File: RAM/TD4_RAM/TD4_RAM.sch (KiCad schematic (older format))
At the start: 1 part, among them U1 74AHC1G32

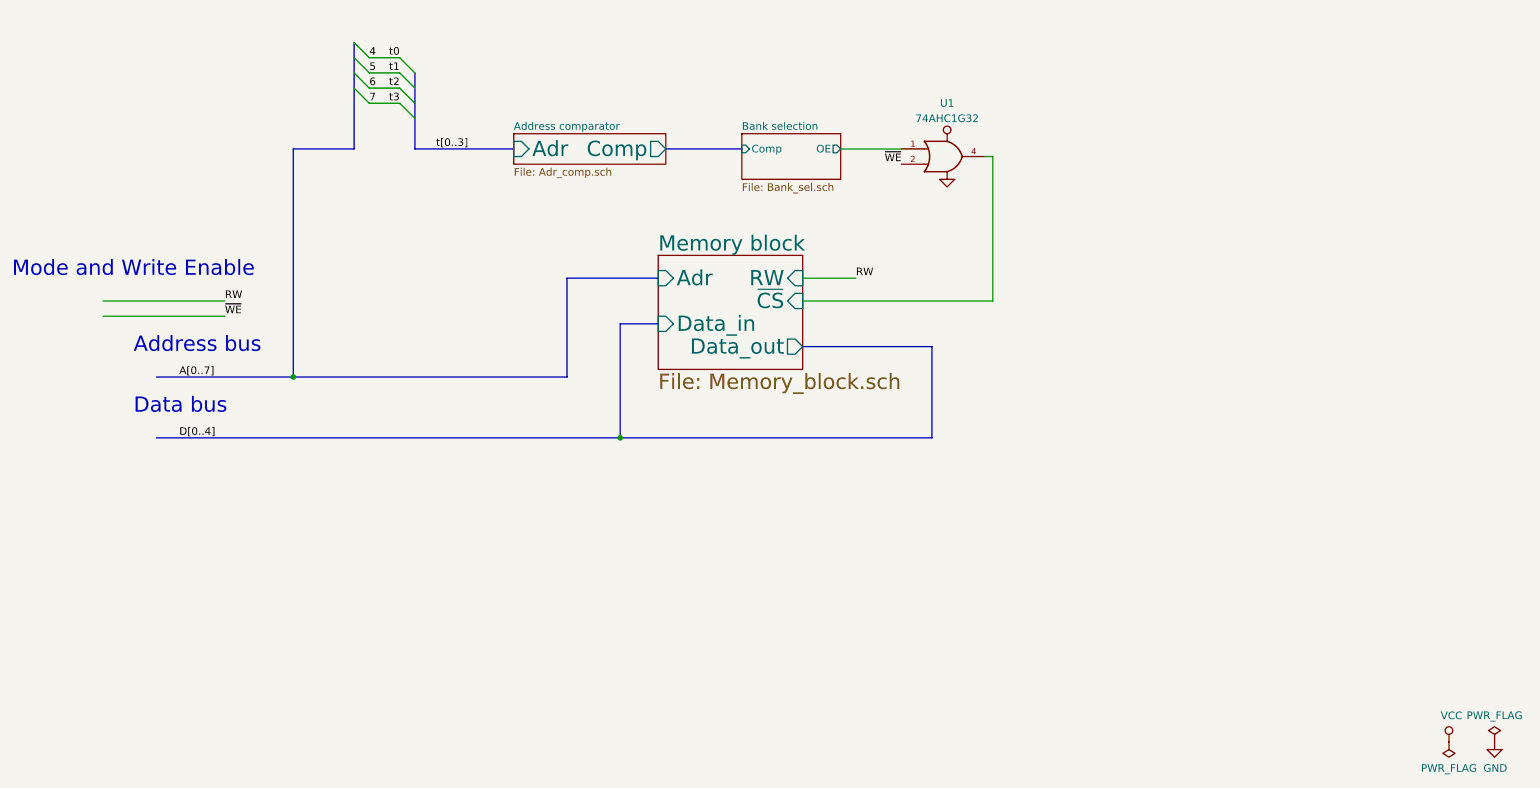
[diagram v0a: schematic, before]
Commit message: RAM done (damn buses\!)
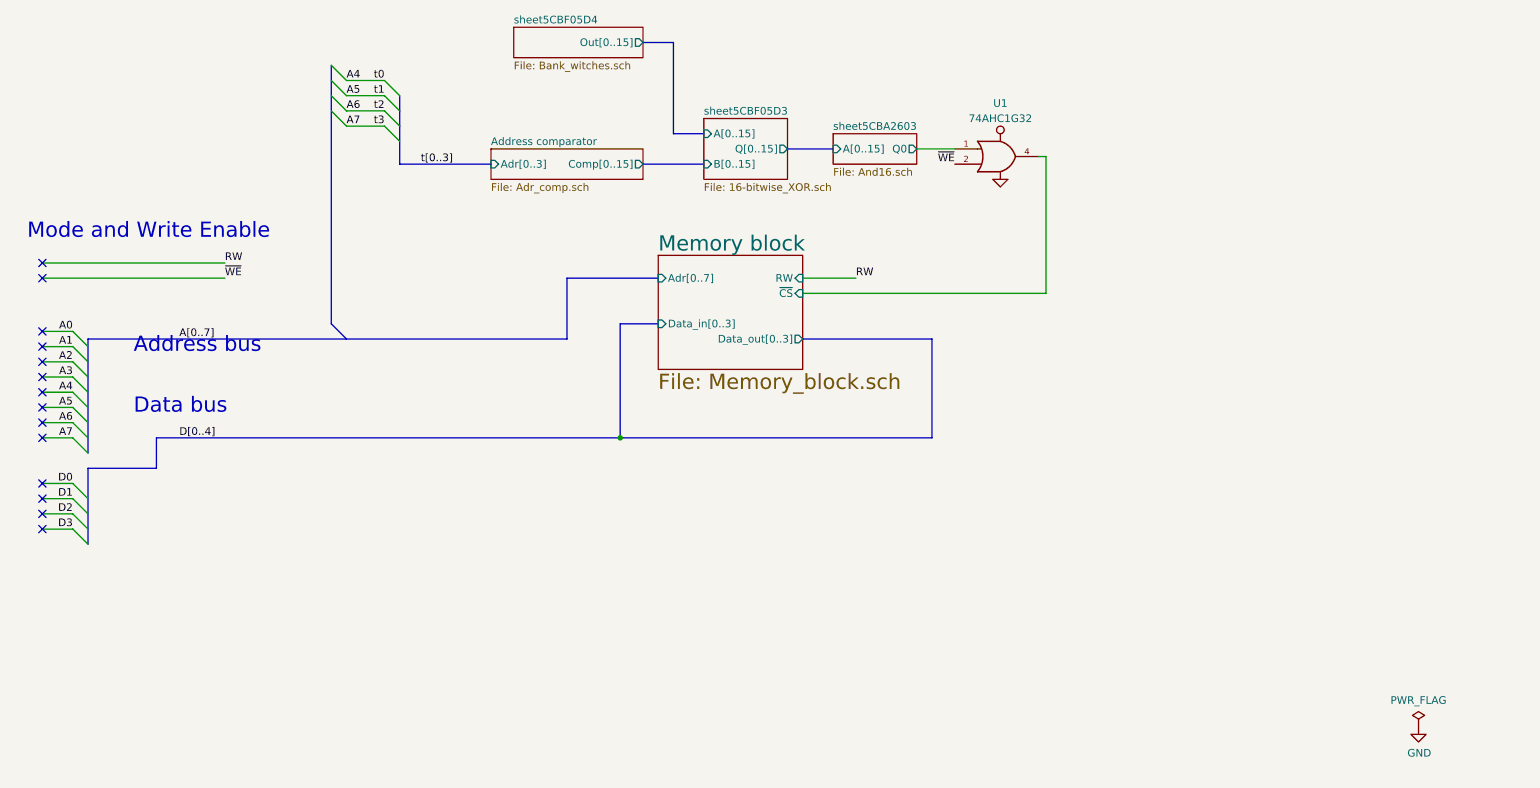
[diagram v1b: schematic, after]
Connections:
- net labels added: A0, A1, A2, A3, A4, A5, A6, A7, D0, D1, D2, D3
- net labels removed: 4, 5, 6, 7
- wire segments 11 -> 23
- no-connect marks 0 -> 14
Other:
- moved on the sheet: U1
